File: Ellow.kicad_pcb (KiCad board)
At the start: 2 copper layers, 20.8 x 36.5 mm, 23 parts, among them J1 USB_C_Receptacle_USB2.0, J2 M_2_AKey_KB, J3 Conn_01x02_Female, Q1 A03407, Q2 A03407, U1 AP2112K-3.3, U2 E73-2G4M08S1C, U3 LN2054Y42AMR

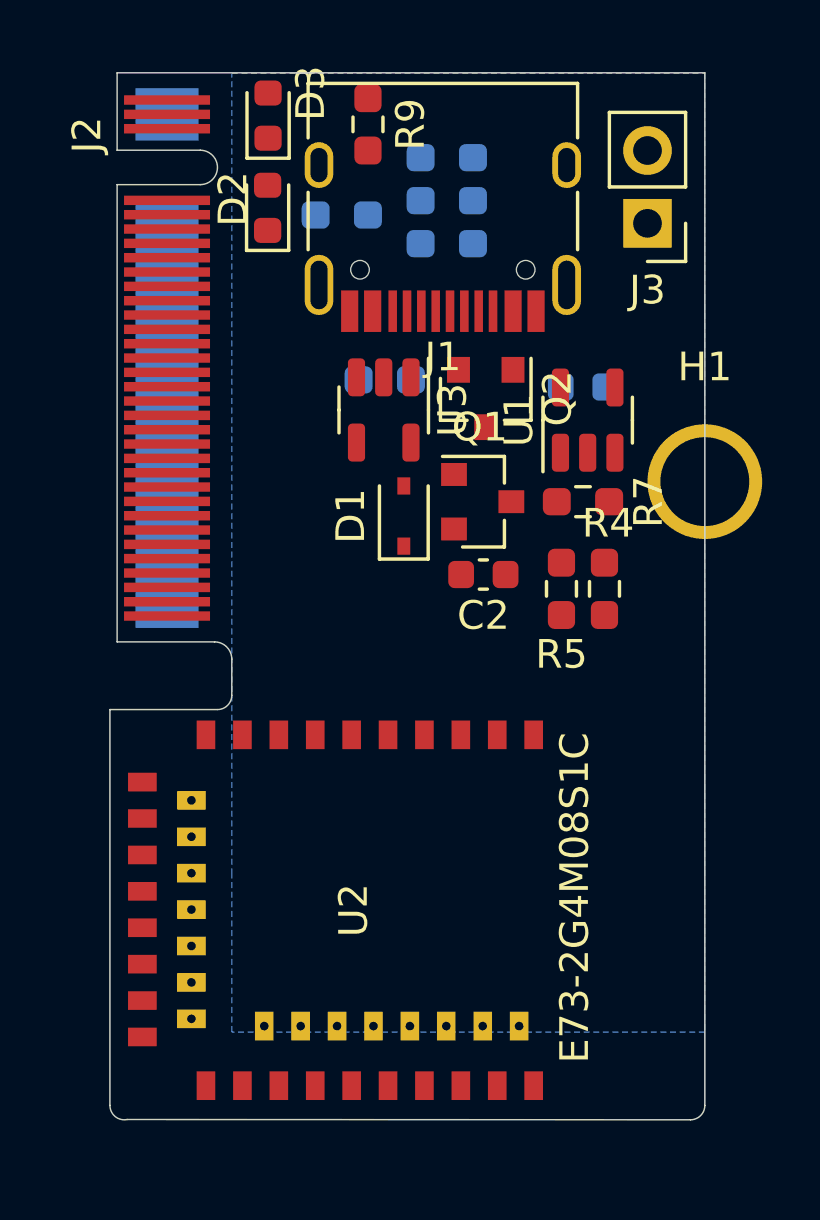
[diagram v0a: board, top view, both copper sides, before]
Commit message: prelim routing
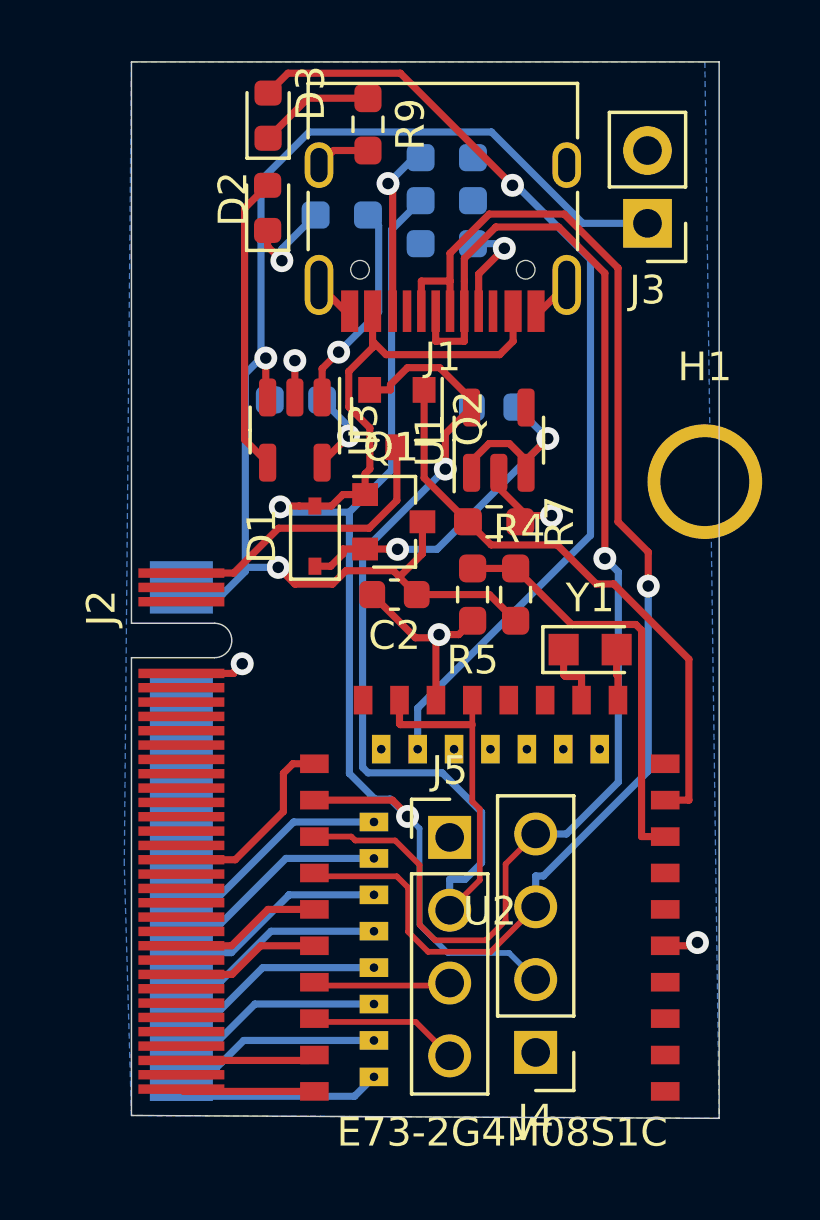
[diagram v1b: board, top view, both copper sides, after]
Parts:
- added J4: Conn_01x04_Female, ellow:PinHeader_1x04_P2.54mm_Vertical_small, F.Cu at (239.4, 127.1)
- added J5: Conn_01x04_Female, ellow:PinHeader_1x04_P2.54mm_Vertical_small, F.Cu at (236.4, 119.6)
- added Y1: 32.768kHz, Crystal:Crystal_SMD_2012-2Pin_2.0x1.2mm_HandSoldering, F.Cu at (241.3, 113.1)
- moved J2 16.5 mm to (225.3, 119.4)
- moved U2 14.7 mm to (237.8, 114.4), turned to 270 degrees
- moved C1 3.18 mm to (237.9, 104.6)
- moved C2 3.18 mm to (234.5, 111.1)
- moved D1 3.18 mm to (231.7, 109.1)
- moved Q1 3.18 mm to (234.4, 108.6)
- moved R7 3.18 mm to (237.9, 108.6)
- moved U1 3.18 mm to (238.1, 105.8)
- moved U3 3.18 mm to (231.0, 105.4)
- moved Q2 3.18 mm to (234.5, 105.0)
- moved R8 3.18 mm to (231.0, 104.4)
- moved R4 3.11 mm to (238.7, 111.1)
- moved R5 3.11 mm to (237.2, 111.1)
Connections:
- D3 pad 2: Net-(D3-Pad2) -> P0.07
- J2 pad 16: P0.31 -> GND
- J2 pad 17: P0.30 -> GND
- J2 pad 20: P0.29 -> Net-(J2-Pad20)
- J2 pad 21: P0.02 -> Net-(J2-Pad21)
- J2 pad 24: P1.13 -> Net-(J2-Pad24)
- J2 pad 25: GND -> Net-(J2-Pad25)
- J2 pad 28: P0.03 -> Net-(J2-Pad28)
- J2 pad 29: P0.28 -> Net-(J2-Pad29)
- J2 pad 32: P1.11 -> Net-(J2-Pad32)
- J2 pad 33: P1.06 -> Net-(J2-Pad33)
- J2 pad 36: P0.10 -> Net-(J2-Pad36)
- J2 pad 37: P0.09 -> Net-(J2-Pad37)
- J2 pad 40: GND -> Net-(J2-Pad40)
- J2 pad 41: P0.24 -> Net-(J2-Pad41)
- J2 pad 42: Net-(J2-Pad42) -> RESET
- J2 pad 44: P0.13 -> Net-(J2-Pad44)
- J2 pad 45: P0.20 -> Net-(J2-Pad45)
- J2 pad 47: Net-(J2-Pad47) -> P0.15
- J2 pad 48: P0.17 -> Net-(J2-Pad48)
- J2 pad 49: P0.15 -> Net-(J2-Pad49)
- J2 pad 51: Net-(J2-Pad51) -> P0.17
- J2 pad 52: P0.08 -> Net-(J2-Pad52)
- J2 pad 53: GND -> Net-(J2-Pad53)
- J2 pad 54: Net-(J2-Pad54) -> P0.13
- J2 pad 55: Net-(J2-Pad55) -> P0.20
- J2 pad 58: Net-(J2-Pad58) -> P0.24
- J2 pad 59: Net-(J2-Pad59) -> P0.22
- J2 pad 6: RESET -> Net-(J2-Pad6)
- J2 pad 63: Net-(J2-Pad63) -> P1.00
- J2 pad 67: Net-(J2-Pad67) -> P1.02
- J2 pad 70: Net-(J2-Pad70) -> P0.09
- J2 pad 71: Net-(J2-Pad71) -> P1.04
- J2 pad 74: Net-(J2-Pad74) -> P0.10
- J2 pad 75: Net-(J2-Pad75) -> P1.06
- U2 pad 10: P0.30 -> PROG
- U2 pad 15: PROG -> Net-(U2-Pad15)
- U2 pad 17: EXT_VCC_CONTROL -> Net-(U2-Pad17)
- U2 pad 18: BATTERY_MEASURE -> Net-(U2-Pad18)
- U2 pad 2: Net-(D3-Pad2) -> Net-(U2-Pad2)
- U2 pad 22: 90.07 -> P0.07
- U2 pad 8: P0.29 -> BATTERY_MEASURE
- U2 pad 9: P0.31 -> EXT_VCC_CONTROL
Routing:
- net VBUS: track 0.00 -> 55.3 mm, vias 0 -> 2
- net VBAT: track 0.00 -> 46.4 mm, vias 0 -> 2
- net DATA+: track 0.00 -> 46.2 mm, vias 0 -> 1
- net DATA-: track 0.00 -> 45.7 mm, vias 0 -> 1
- net VDD_H: track 0.00 -> 39.1 mm, vias 0 -> 1
- net P0.07: track 0.00 -> 33.8 mm, vias 0 -> 1
- net EXT_VCC_CONTROL: track 0.00 -> 20.7 mm
- net GND: track 0.00 -> 19.2 mm, vias 0 -> 5
- net Net-(C1-Pad1): track 0.00 -> 15.9 mm, vias 0 -> 2
- net BATTERY_MEASURE: track 0.00 -> 14.8 mm
- net EXT_VCC: track 0.00 -> 10.4 mm
- net Net-(D2-Pad2): track 0.00 -> 10.3 mm
- net P0.15: track 0.00 -> 7.78 mm
- net P0.17: track 0.00 -> 7.67 mm
- net P0.20: track 0.00 -> 7.56 mm
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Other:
- board size 20.8 x 36.5 mm -> 20.5 x 36.8 mm
